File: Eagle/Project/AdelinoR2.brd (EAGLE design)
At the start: 47 x 53.3 mm, 80 parts, among them J1 DC-044-A, J2 YELLOW-8P-2.54, J3 YELLOW-6P-2.54, J4 YELLOW-8P-2.54, J5 YELLOW-8P-2.54, J6 4P-2.0, J7 YELLOW-2X3P-2.54, J8 4P-2.0, Q1 NCE3407A, Q2 CJ2305, SW1 TS-1101F, U1 CJT1117-3.3-SOT223, U2 MP1496DJ-SOT23-8, U3 ESP-12F / OPL: 317060163 / SM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, U4 ATMEGA32U4-MUR-QFN44, U5 ATMEGA32U4-TQFP44, U6 ATECC608-SOIC8, X1 306010049_XTAL_16MHZ-3225_4P

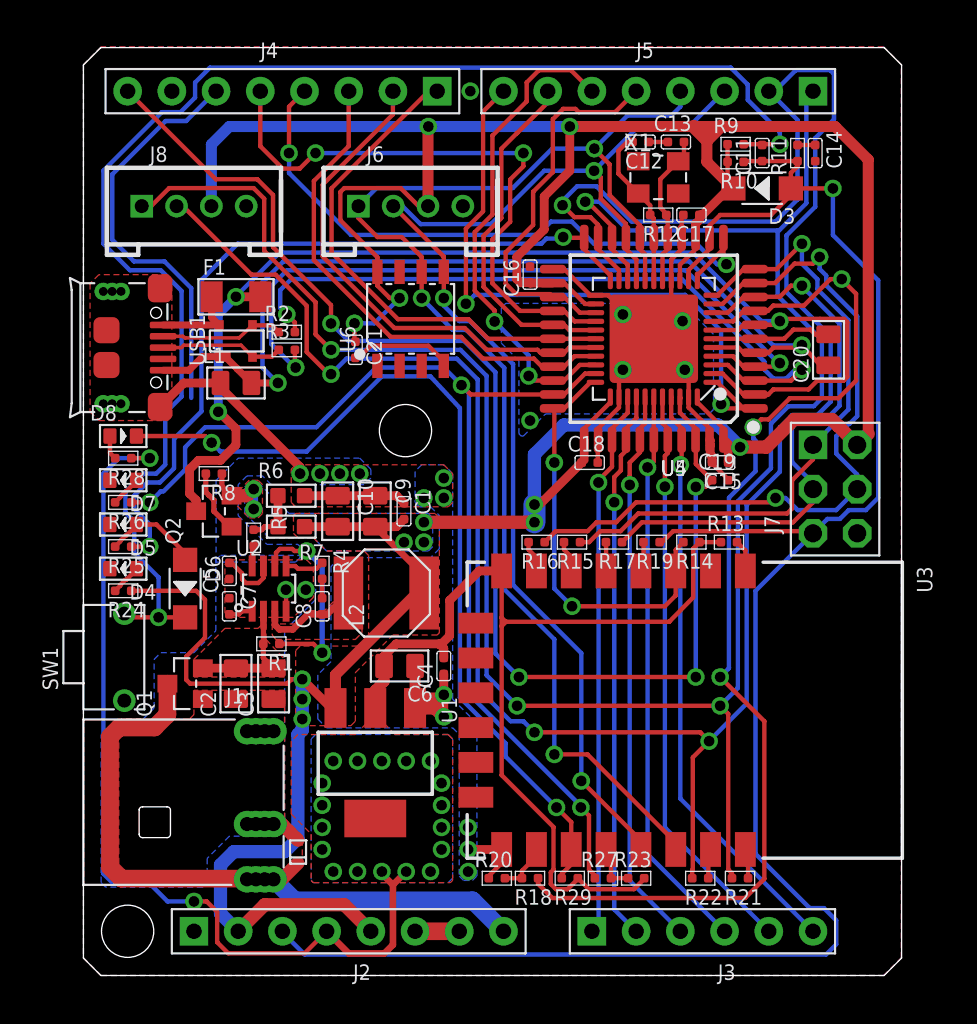
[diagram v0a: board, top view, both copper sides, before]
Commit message: Routing wip.
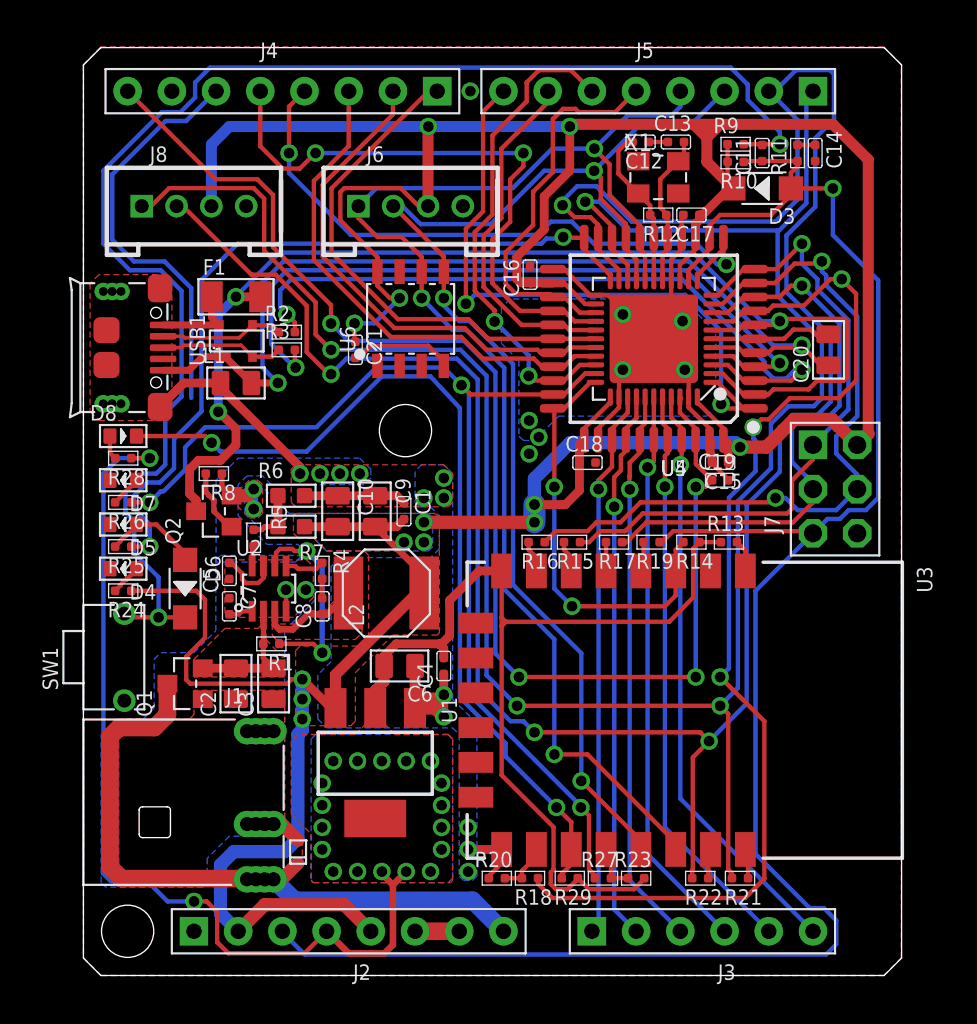
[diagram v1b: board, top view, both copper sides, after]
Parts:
- moved C18 0.13 mm to (29.0, 29.5)
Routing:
- net GND: track 81.4 -> 80.3 mm, vias 20 -> 22
- net +5V: track 227.5 -> 226.9 mm
